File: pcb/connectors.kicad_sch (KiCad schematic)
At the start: 7 parts, among them J1 GT-USB-7010, J6 KF350-3.5-2P, U1 USBLC6-2P6

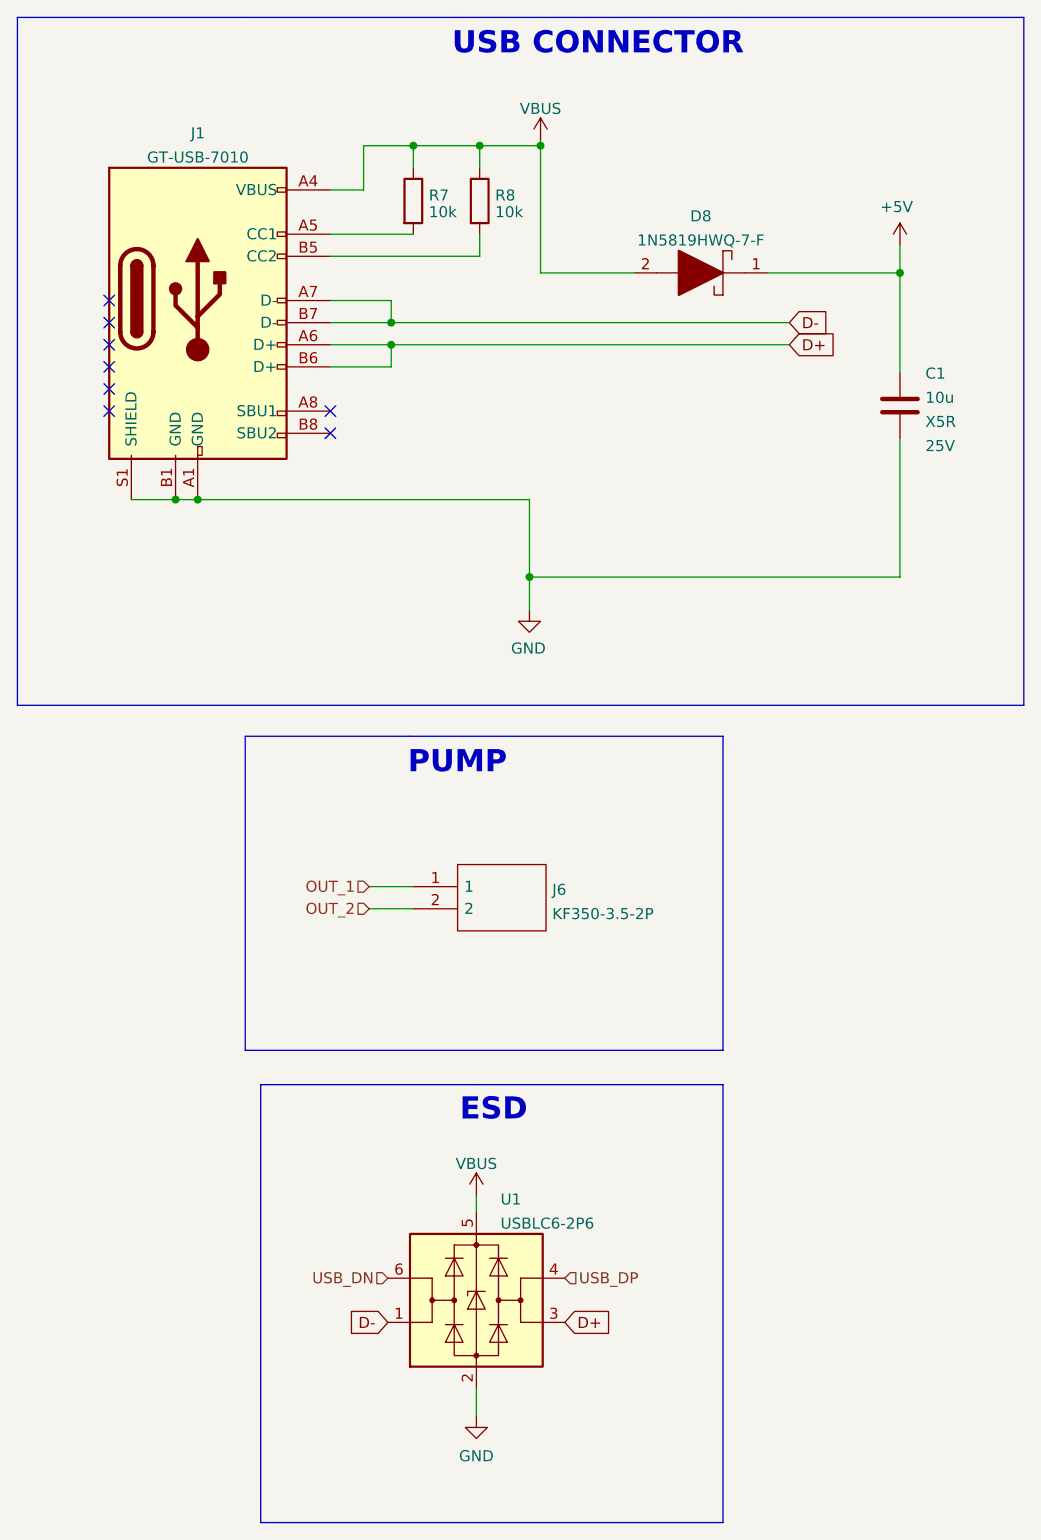
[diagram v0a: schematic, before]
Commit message: created step file
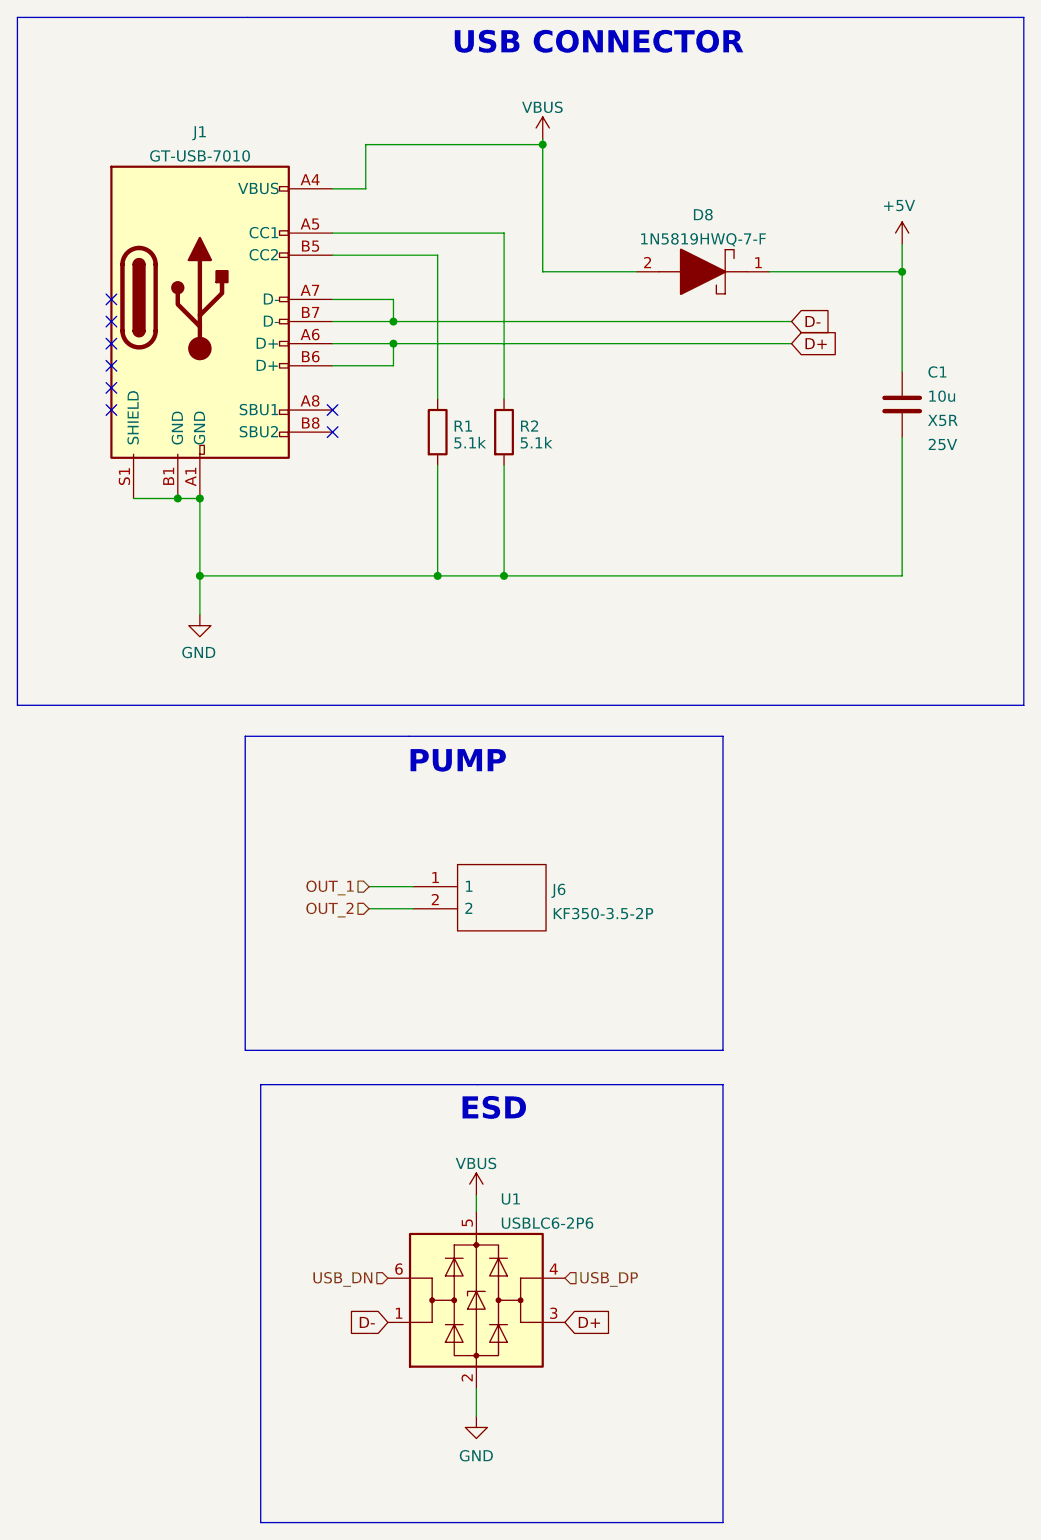
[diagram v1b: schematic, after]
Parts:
- removed R7, R8: 10k, Resistor_SMD:R_0402_1005Metric, symbol Resistor_JLC:10k
- added R1, R2: 5.1k, Resistor_SMD:R_0402_1005Metric, symbol Resistor_JLC:5.1k
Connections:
- net GND: now also R1.2, R2.2
- net at J1.A5 (CC1): now also R2.1
- net at J1.B5 (CC2): now also R1.1
